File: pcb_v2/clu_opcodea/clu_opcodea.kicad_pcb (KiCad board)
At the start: 2 copper layers, 43.2 x 41.4 mm, 54 parts, among them J1 UCODE, U1 74LS00

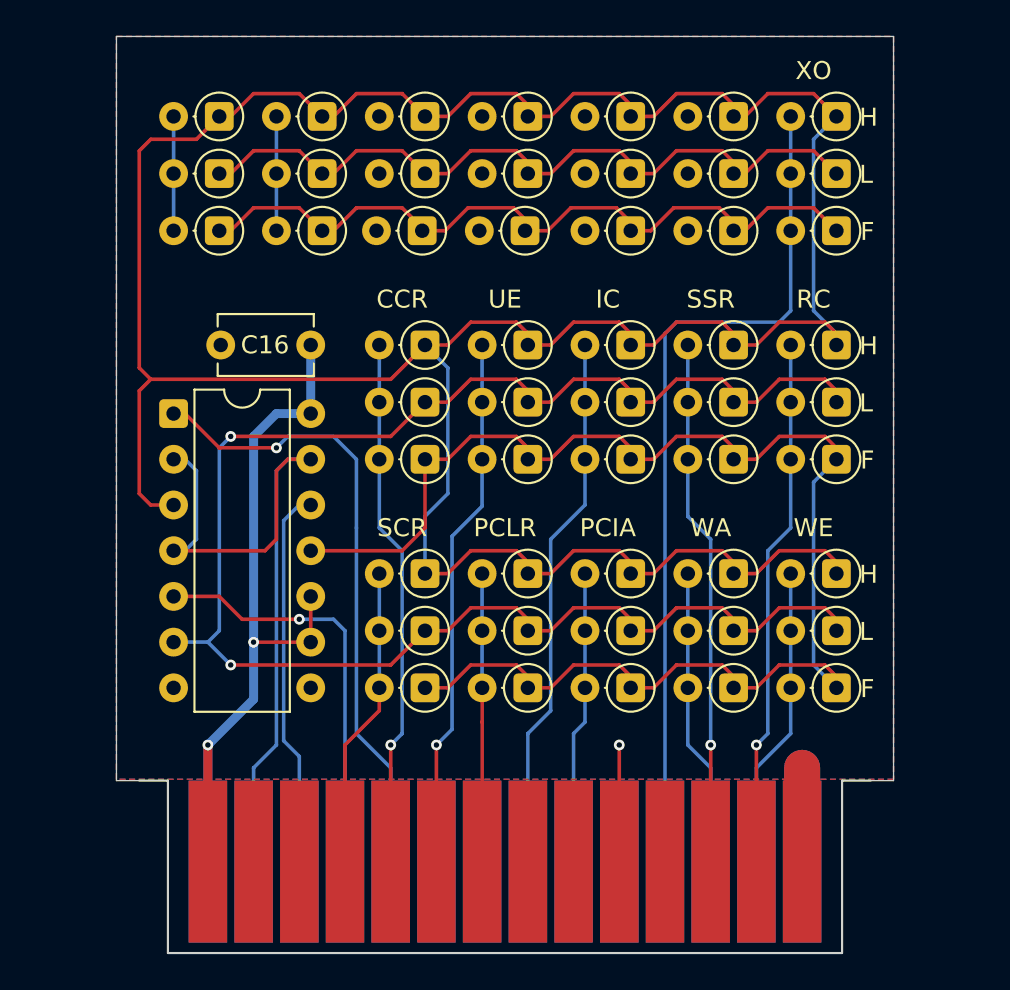
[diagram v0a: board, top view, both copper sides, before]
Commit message: alteração de layout
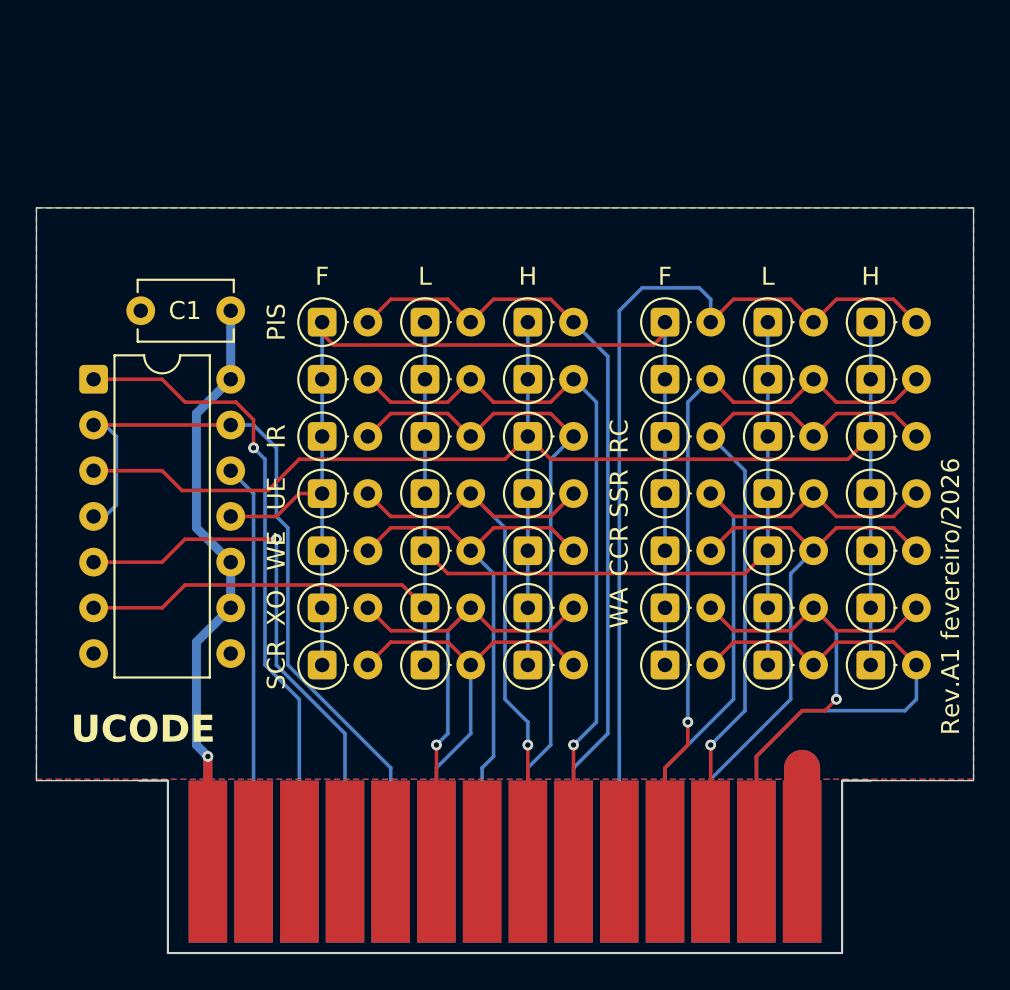
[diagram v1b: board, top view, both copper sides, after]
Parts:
- removed D43, D44, D45, D46, D47, D48, D49, D50, D51: 1N4148, Diode_THT:D_DO-35_SOD27_P2.54mm_Vertical_AnodeUp
- moved D31 35.4 mm to (61.0, 74.9), turned to 0 degrees
- moved D32 33.2 mm to (66.7, 74.9), turned to 0 degrees
- moved D33 32.2 mm to (72.4, 74.9), turned to 0 degrees
- moved D1 29.6 mm to (61.0, 71.8), turned to 0 degrees
- moved D27 27.3 mm to (91.4, 71.8), turned to 0 degrees
- moved D7 26.6 mm to (61.0, 59.1), turned to 0 degrees
- moved D2 23.3 mm to (66.7, 71.8), turned to 0 degrees
- moved D42 22.2 mm to (91.4, 59.1), turned to 0 degrees
- moved D26 20.8 mm to (85.7, 71.8), turned to 0 degrees
- moved D8 20.6 mm to (66.7, 59.1), turned to 0 degrees
- moved D12 19.7 mm to (91.4, 78.1), turned to 0 degrees
- moved D37 19.0 mm to (61.0, 62.2), turned to 0 degrees
- moved D22 17.2 mm to (61.0, 65.4), turned to 0 degrees
- moved D3 17.2 mm to (72.4, 71.8), turned to 0 degrees
- moved D36 16.5 mm to (91.4, 62.2), turned to 0 degrees
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- renumbered C16 to C1
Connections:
- D10 pad 2: ~{UC_pclr_swap} -> ~{UC_D}
- D11 pad 2: ~{UC_pclr_swap} -> ~{UC_D}
- D12 pad 2: ~{UC_pclr_swap} -> ~{UC_D}
- D34 pad 2: ~{UC_F} -> ~{UC_C}
- D35 pad 2: ~{UC_F} -> ~{UC_C}
- D36 pad 2: ~{UC_F} -> ~{UC_C}
- D37 pad 2: ~{UC_E} -> ~{UC_B}
- D38 pad 2: ~{UC_E} -> ~{UC_B}
- D39 pad 2: ~{UC_E} -> ~{UC_B}
- D40 pad 2: ~{UC_D} -> ~{UC_A}
- D41 pad 2: ~{UC_D} -> ~{UC_A}
- D42 pad 2: ~{UC_D} -> ~{UC_A}
- J1 pad 10: ~{UC_F} -> unconnected-(J1-Pin_10-Pad10)
- J1 pad 11: unconnected-(J1-Pin_11-Pad11) -> ~{UC_C}
- J1 pad 12: ~{UC_save_src_reg} -> ~{UC_restart_cycle}
- J1 pad 13: ~{UC_restart_cycle} -> ~{UC_write_address}
- J1 pad 16: select_opcode -> fetch_cycle
- J1 pad 17: fetch_cycle -> high_cycle
- J1 pad 19: high_cycle -> select_opcode
- J1 pad 2: ~{UC_A} -> unconnected-(J1-Pin_2-Pad2)
- J1 pad 20: ~{UC_D} -> ~{UC_save_cond_reg}
- J1 pad 21: unconnected-(J1-Pin_21-Pad21) -> ~{UC_write_enable}
- J1 pad 24: unconnected-(J1-Pin_24-Pad24) -> ~{UC_A}
- J1 pad 25: ~{UC_extended_opcode} -> ~{UC_save_src_reg}
- J1 pad 26: ~{UC_write_address} -> ~{UC_clear_cond_reg}
- J1 pad 27: ~{UC_write_enable} -> ~{UC_D}
- J1 pad 3: ~{UC_E} -> unconnected-(J1-Pin_3-Pad3)
- J1 pad 4: ~{UC_save_cond_reg} -> unconnected-(J1-Pin_4-Pad4)
- J1 pad 5: ~{UC_clear_cond_reg} -> unconnected-(J1-Pin_5-Pad5)
- J1 pad 6: ~{UC_ula_enable} -> ~{UC_extended_opcode}
- J1 pad 7: ~{UC_pclr_swap} -> unconnected-(J1-Pin_7-Pad7)
- J1 pad 8: ~{UC_C} -> ~{UC_ula_enable}
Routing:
- net Net-(D1-K): track 161.2 -> 64.6 mm
- net Net-(D12-K): track 174.4 -> 84.0 mm
- net ~{UC_A}: track 6.35 -> 51.3 mm
- net ~{UC_C}: track 0.00 -> 41.4 mm, vias 0 -> 1
- net ~{UC_B}: track 6.35 -> 41.4 mm, vias 0 -> 1
- net ~{UC_D}: track 0.00 -> 31.5 mm
- net ~{UC_pcia_swap}: track 16.3 -> 45.1 mm
- net Net-(D11-K): track 101.3 -> 77.7 mm, vias 2 -> 0
- net ~{UC_extended_opcode}: track 47.6 -> 28.4 mm, vias 0 -> 1
- net ~{UC_pclr_swap}: track 16.0 -> 0.00 mm
- net ~{UC_write_enable}: track 16.8 -> 31.6 mm
- net ~{UC_write_address}: track 16.5 -> 30.7 mm, vias 0 -> 1
- net ~{UC_restart_cycle}: track 29.5 -> 38.7 mm
- net ~{UC_save_cond_reg}: track 16.8 -> 25.2 mm
- net ~{UC_int_ready}: track 30.0 -> 38.2 mm
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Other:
- board size 43.2 x 41.4 mm -> 52.1 x 31.8 mm
- board text added: "IR"
- board text added: "PIS"
- board text added: "Rev.A1 fevereiro/2026"
- board text added: "UCODE"
- board text removed: "IC"
- board text removed: "PCIA"
- board text removed: "PCLR"
